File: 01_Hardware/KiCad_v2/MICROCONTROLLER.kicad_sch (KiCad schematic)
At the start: 33 parts, among them Q500 IRLML2402TRPBF, U500 DS3231M, U501 ESP32-WROOM-32E-N4, U502 AT24CS01-SSHM

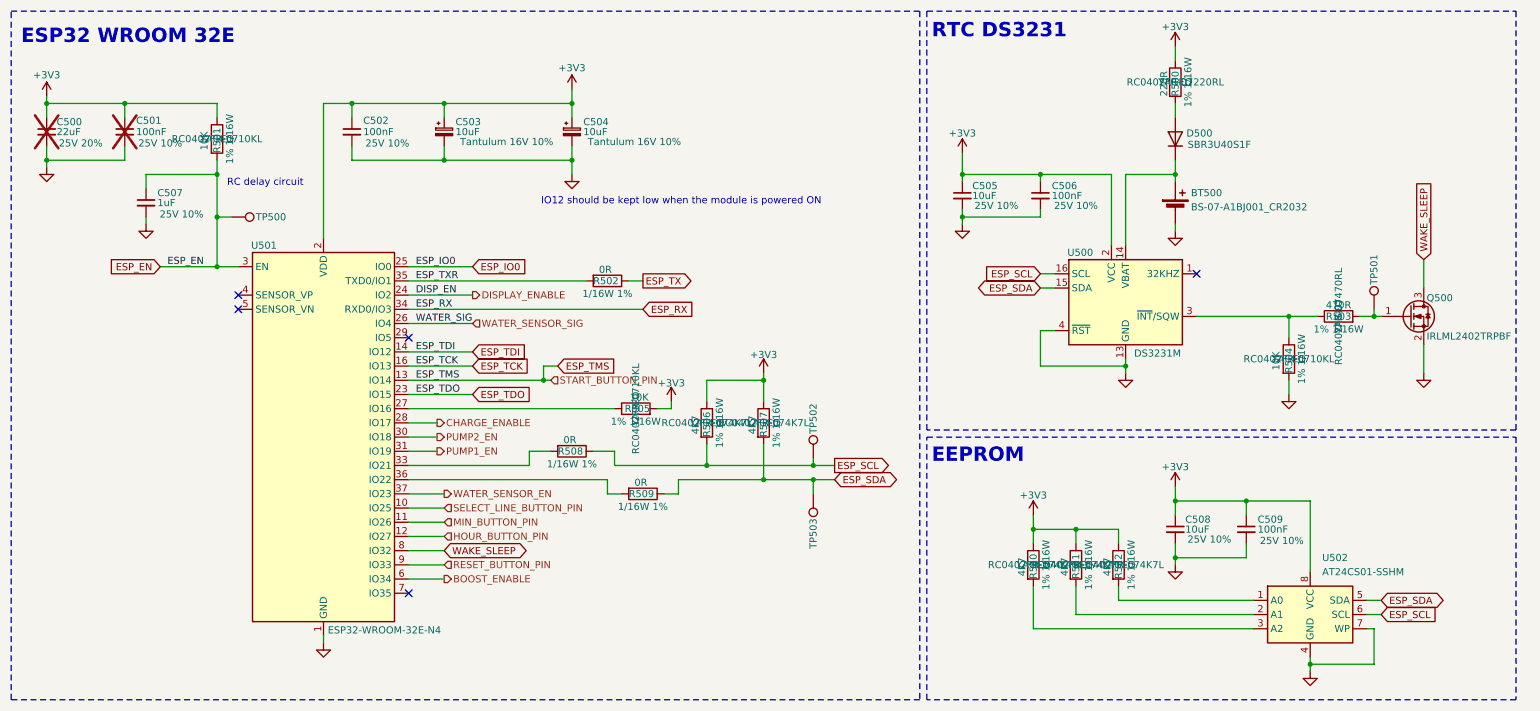
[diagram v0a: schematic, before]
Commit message: USB-C and Serial PCB routing done
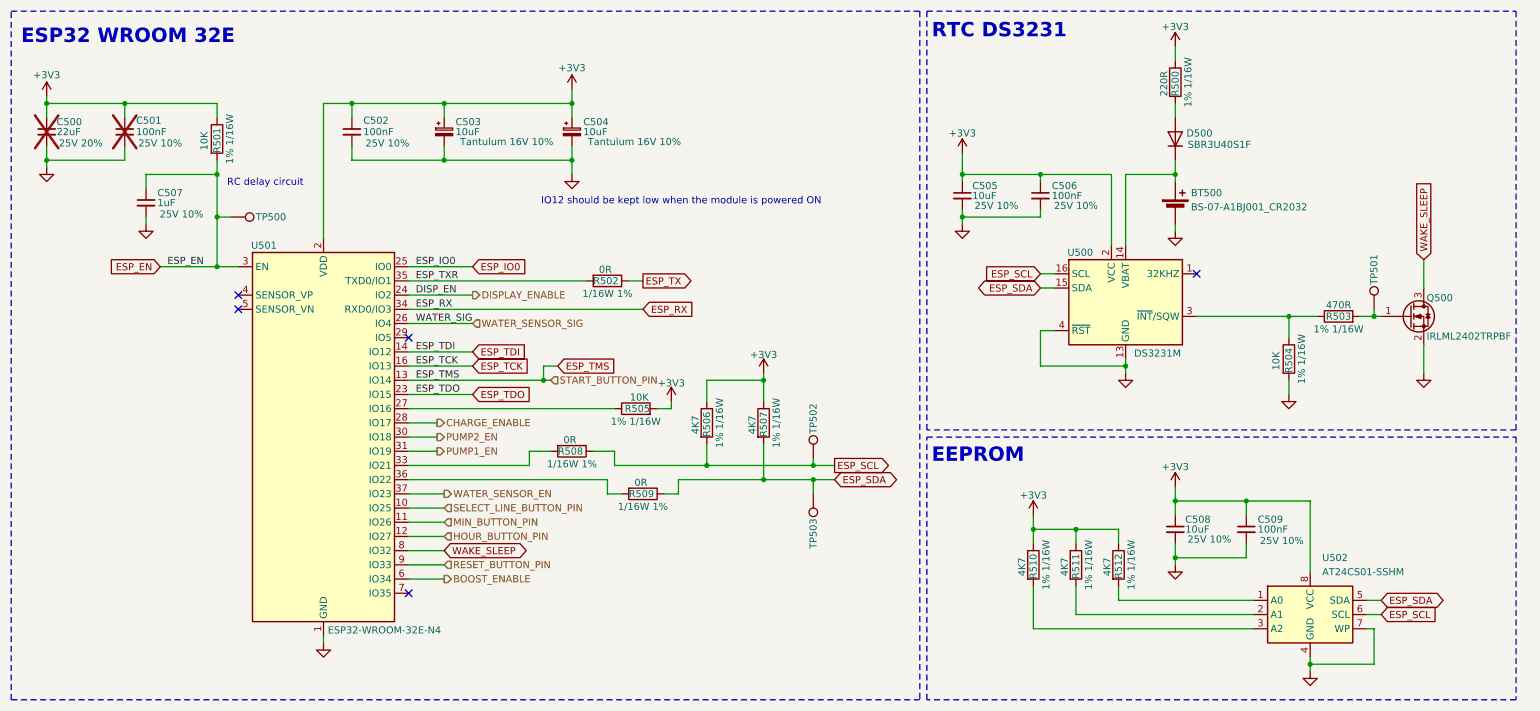
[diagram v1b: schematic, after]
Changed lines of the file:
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@@
 					(size 1.27 1.27)
 				)
+				(hide yes)
 			)
 		)
@@
 					(size 1.27 1.27)
 				)
+				(hide yes)
 			)
 		)
@@
 					(size 1.27 1.27)
 				)
+				(hide yes)
 			)
 		)
@@
 					(size 1.27 1.27)
 				)
+				(hide yes)
 			)
 		)
@@
 					(size 1.27 1.27)
 				)
+				(hide yes)
 			)
 		)
@@
 					(size 1.27 1.27)
 				)
+				(hide yes)
 			)
 		)
@@
 					(size 1.27 1.27)
 				)
+				(hide yes)
 			)
 		)
@@
 					(size 1.27 1.27)
 				)
+				(hide yes)
 			)
 		)
@@
 					(size 1.27 1.27)
 				)
+				(hide yes)
 			)
 		)
@@
 					(size 1.27 1.27)
 				)
+				(hide yes)
 			)
 		)
@@
 					(size 1.27 1.27)
 				)
+				(hide yes)
 			)
 		)
@@
 					(size 1.27 1.27)
 				)
+				(hide yes)
 			)
 		)
@@
 					(size 1.27 1.27)
 				)
+				(hide yes)
 			)
 		)
@@
 					(size 1.27 1.27)
 				)
+				(hide yes)
 			)
 		)
@@
 					(size 1.27 1.27)
 				)
+				(hide yes)
 			)
 		)
@@
 					(size 1.27 1.27)
 				)
+				(hide yes)
 			)
 		)
@@
 					(size 1.27 1.27)
 				)
+				(hide yes)
 			)
 		)
@@
 					(size 1.27 1.27)
 				)
+				(hide yes)
 			)
 		)
@@
 					(size 1.27 1.27)
 				)
+				(hide yes)
 			)
 		)
@@
 					(size 1.27 1.27)
 				)
+				(hide yes)
 			)
 		)
@@
 					(size 1.27 1.27)
 				)
+				(hide yes)
 			)
 		)
@@
 					(size 1.27 1.27)
 				)
+				(hide yes)
 			)
 		)
@@
 					(size 1.27 1.27)
 				)
+				(hide yes)
 			)
 		)
@@
 					(size 1.27 1.27)
 				)
+				(hide yes)
 			)
 		)
@@
 					(size 1.27 1.27)
 				)
+				(hide yes)
 			)
 		)
@@
 					(size 1.27 1.27)
 				)
+				(hide yes)
 			)
 		)
@@
 					(size 1.27 1.27)
 				)
+				(hide yes)
 			)
 		)
@@
 					(size 1.27 1.27)
 				)
+				(hide yes)
 			)
 		)
@@
 					(size 1.27 1.27)
 				)
+				(hide yes)
 			)
 		)
@@
 					(size 1.27 1.27)
 				)
+				(hide yes)
 			)
 		)
@@
 					(size 1.27 1.27)
 				)
+				(hide yes)
 			)
 		)
@@
 					(size 1.27 1.27)
 				)
+				(hide yes)
 			)
 		)
@@
 					(size 1.27 1.27)
 				)
+				(hide yes)
 			)
 		)
@@
 					(size 1.27 1.27)
 				)
+				(hide yes)
 			)
 		)
@@
 					(size 1.27 1.27)
 				)
+				(hide yes)
 			)
 		)
@@
 					(size 1.27 1.27)
 				)
+				(hide yes)
 			)
 		)
@@
 					(size 1.27 1.27)
 				)
+				(hide yes)
 			)
 		)
@@
 					(size 1.27 1.27)
 				)
+				(hide yes)
 			)
 		)
@@
 					(size 1.27 1.27)
 				)
+				(hide yes)
 			)
 		)
@@
 					(size 1.27 1.27)
 				)
+				(hide yes)
 			)
 		)
